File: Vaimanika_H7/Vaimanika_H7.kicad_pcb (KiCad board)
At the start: 4 copper layers, 40 x 40 mm, 63 parts, among them CN1 WAFER-GH1.25-3PWB, J1 TYPE-C 16PIN 2MD, J2 Conn_01x09, J3 Conn_01x09, J4 +VLIPO, J5 GND, J6 Conn_01x09, J8 Conn_01x02, Q1 AO3400A, Q2 AO3401A, U2 TPS54302, U3 USBLC6-2P6, U4 WAFER-GH1.25-4PWB, U5 WAFER-GH1.25-4PWB, U6 WAFER-GH1.25-4PWB, U7 WAFER-GH1.25-4PLB, U8 WAFER-GH1.25-4PLB, U9 WAFER-GH1.25-4PLB

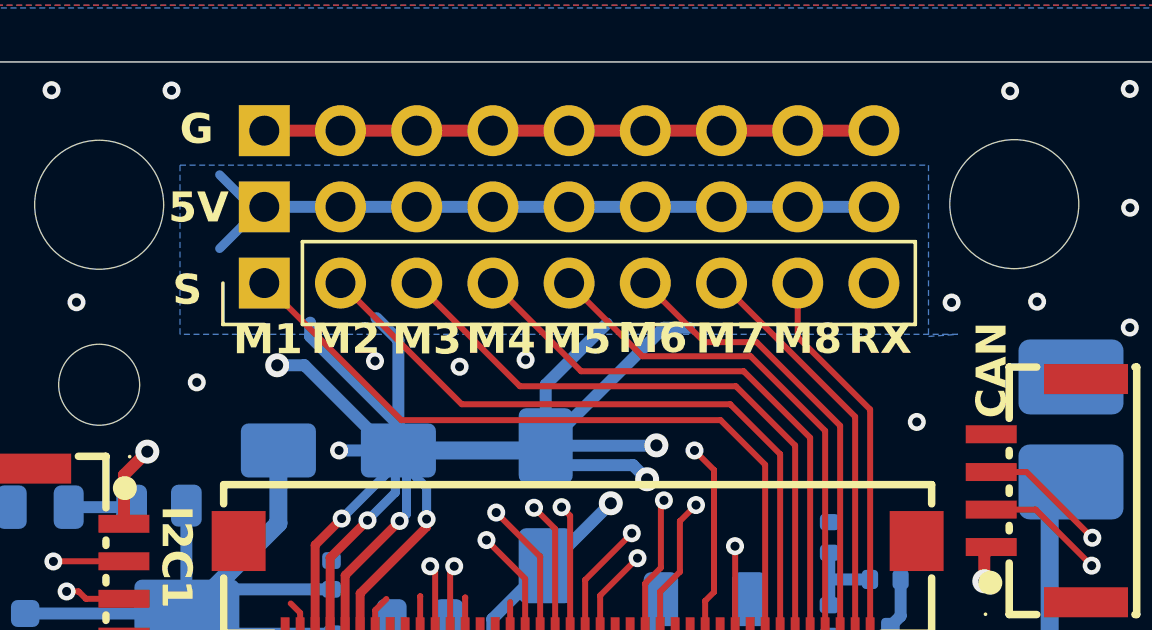
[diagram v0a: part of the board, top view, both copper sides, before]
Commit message: 22-05-2026
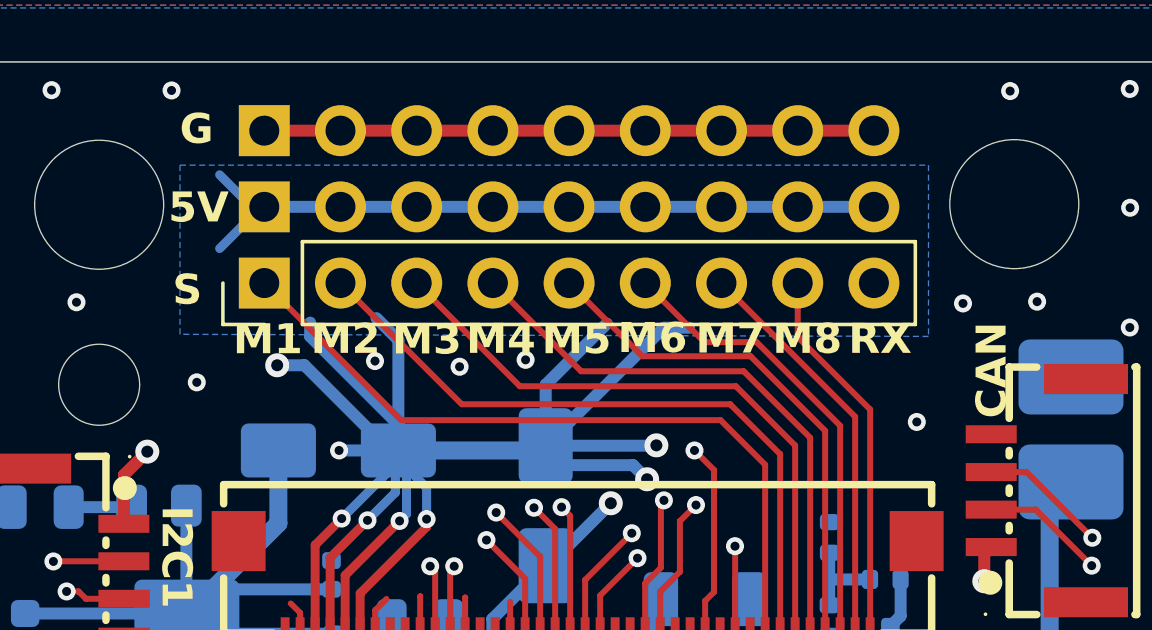
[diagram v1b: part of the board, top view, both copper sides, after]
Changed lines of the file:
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@@
 			)
 		)
-		(property "LCSC" "C492401"
-			(at 0 0 180)
-			(unlocked yes)
-			(layer "F.Fab")
-			(hide yes)
-			(effects
-				(font
-					(size 1 1)
-					(thickness 0.15)
-				)
-			)
-		)
 		(property ki_fp_filters "Connector*:*_1x??_*")
 		(sheetname "/")
@@
 			)
 		)
-		(property "LCSC" "C492408"
-			(at 0 0 90)
-			(unlocked yes)
-			(layer "F.Fab")
-			(hide yes)
-			(effects
-				(font
-					(size 1 1)
-					(thickness 0.15)
-				)
-			)
-		)
 		(property ki_fp_filters "Connector*:*_1x??_*")
 		(sheetname "/")
@@
 			)
 		)
-		(property "LCSC" "C492408"
-			(at 0 0 270)
-			(unlocked yes)
-			(layer "B.Fab")
-			(hide yes)
-			(effects
-				(font
-					(size 1 1)
-					(thickness 0.15)
-				)
-				(justify mirror)
-			)
-		)
 		(property ki_fp_filters "Connector*:*_1x??_*")
 		(sheetname "/")
@@
 			)
 		)
-		(property "LCSC" "C492408"
-			(at 0 0 270)
-			(unlocked yes)
-			(layer "B.Fab")
-			(hide yes)
-			(effects
-				(font
-					(size 1 1)
-					(thickness 0.15)
-				)
-				(justify mirror)
-			)
-		)
 		(property ki_fp_filters "Connector*:*_1x??_*")
 		(sheetname "/")
@@
 	)
 	(via
-		(at 153.14 68.72)
+		(at 153.52 68.75)
 		(size 0.6)
 		(drill 0.3)
@@
 		(polygon
 			(pts
-				(xy 127.42 64.14) (xy 152.37 64.14) (xy 152.37 69.85) (xy 153.35 69.78) (xy 127.42 69.78)
+				(xy 127.42 64.14) (xy 152.37 64.14) (xy 152.37 69.85) (xy 127.42 69.78)
 			)
 		)
